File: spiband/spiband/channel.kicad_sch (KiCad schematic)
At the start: 16 parts, among them J2 Conn_01x06, U10 SN74LVC1T45DBV, U11 SN74LVC1T45DBV, U6 TLV70018_SOT353, U8 SN74LVC1T45DBV, U9 SN74LVC1T45DBV

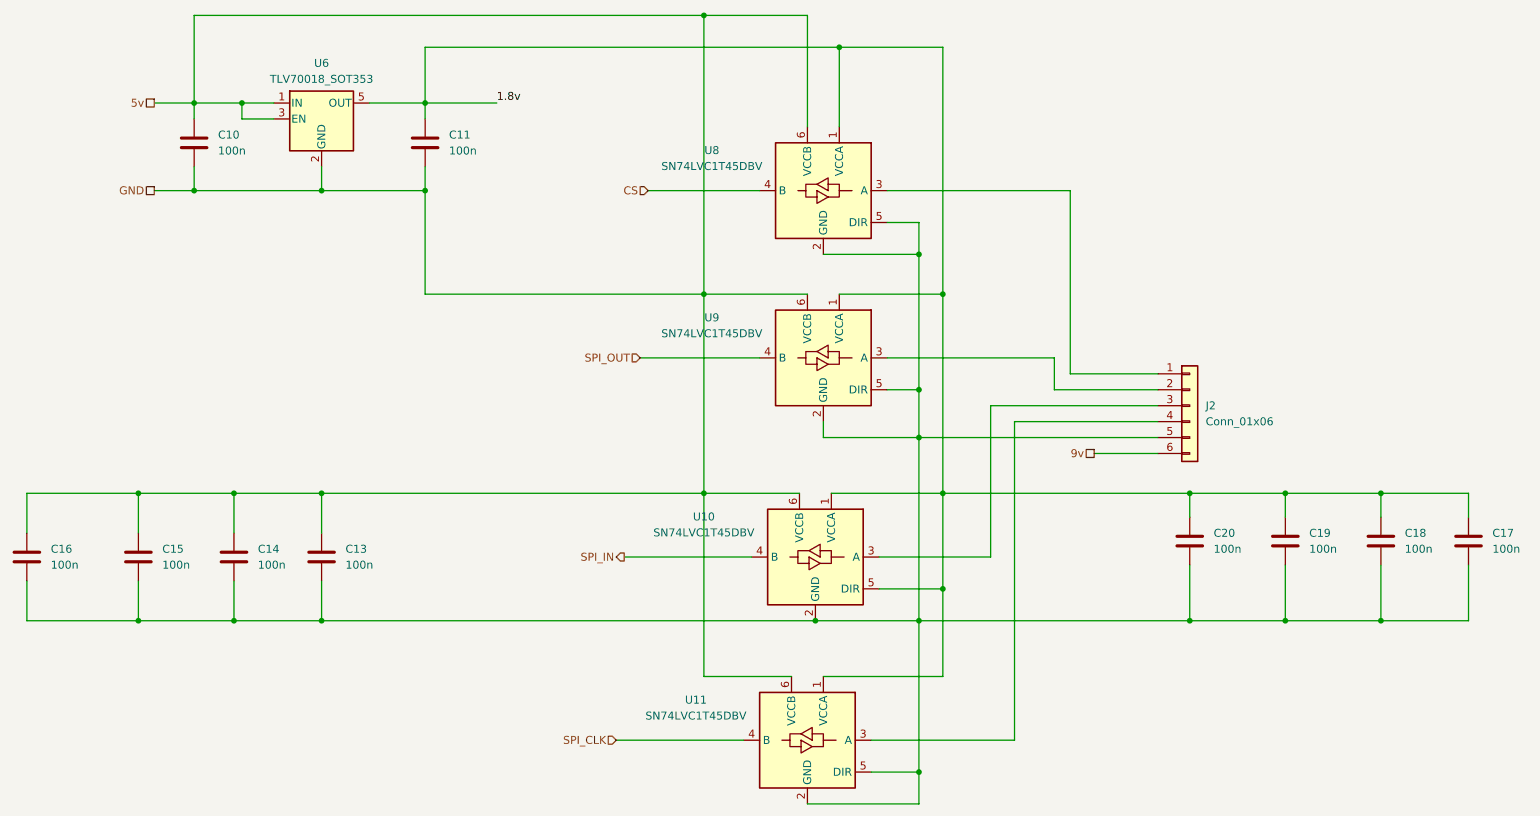
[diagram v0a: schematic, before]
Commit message: SPI band schema done.
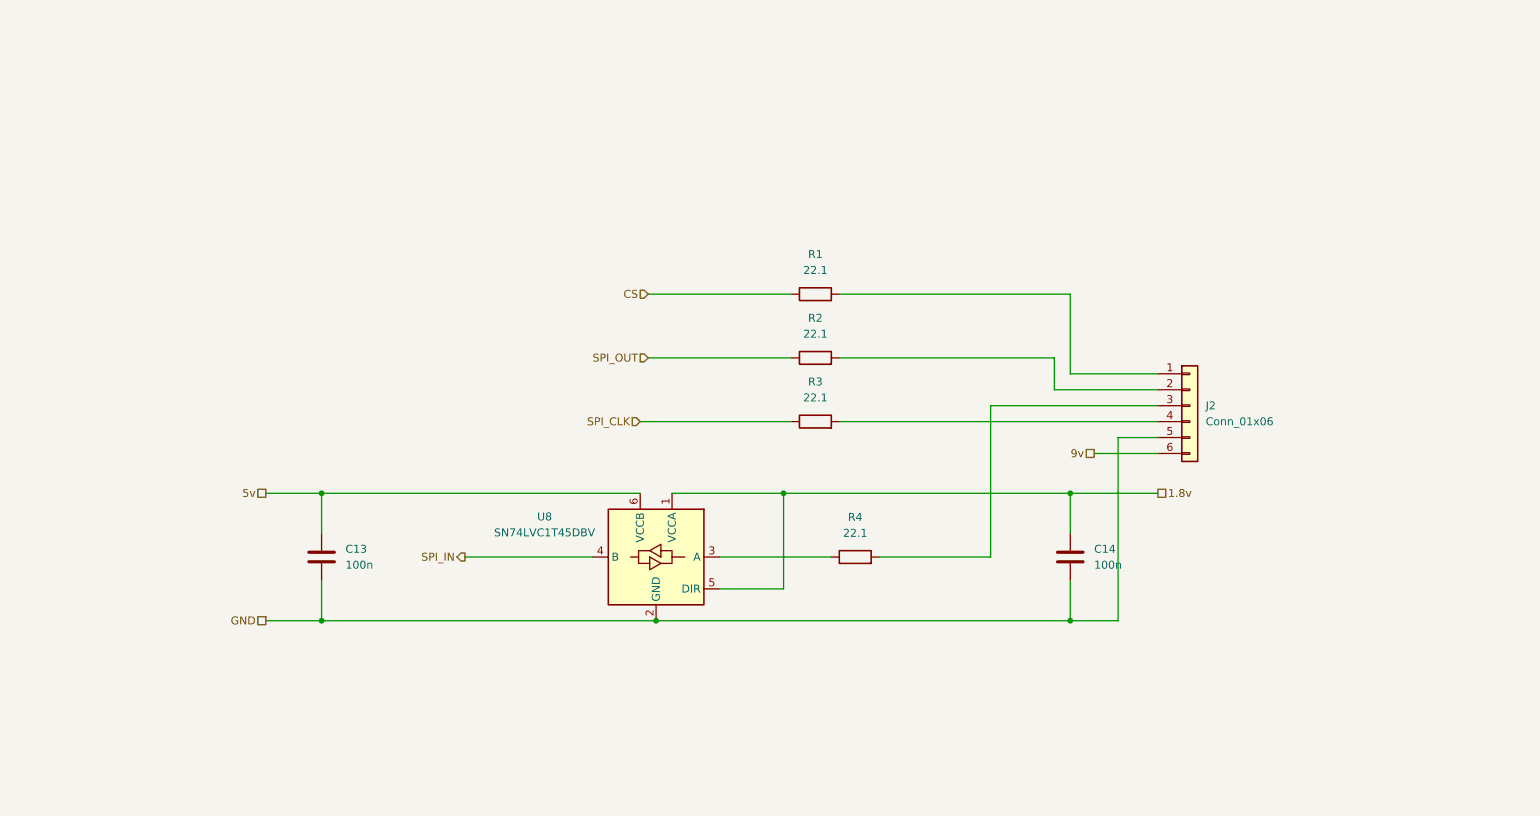
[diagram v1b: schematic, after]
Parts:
- removed C10, C11, C14, C15, C16, C17, C18, C19: 100n, Capacitor_THT:C_Disc_D4.3mm_W1.9mm_P5.00m, symbol Device:C
- removed U11, U8, U9: SN74LVC1T45DBV, Package_TO_SOT_SMD:SOT-23-6, symbol Logic_LevelTranslator:SN74LVC1T45DBV
- removed U6: TLV70018_SOT353, Package_TO_SOT_SMD:SOT-353_SC-70-5, symbol Regulator_Linear:TLV70018_SOT353
- added R1, R2, R3, R4: 22.1, Resistor_SMD:R_0805_2012Metric_Pad1.20x1.40mm_HandSolder, symbol Device:R
- C13: footprint Capacitor_THT:C_Disc_D4.3mm_W1.9mm_P5.00m -> Capacitor_SMD:C_0402_1005Metric_Pad0.74x0.62mm_HandSolder
- C14: renamed from C20; footprint Capacitor_THT:C_Disc_D4.3mm_W1.9mm_P5.00m -> Capacitor_SMD:C_0402_1005Metric_Pad0.74x0.62mm_HandSolder
- renumbered U10 to U8
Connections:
- net CS: now also R1.1
- net SPI_CLK: now also R3.1
- net SPI_OUT: now also R2.1
- net GND: now reaches C13.2, C14.2, J2.5 (Pin_5), U8.2 (GND)
- net at J2.1 (Pin_1): now also R1.2
- net at U8.3 (A): now also R4.1; no longer J2.3 (Pin_3)
- net at J2.2 (Pin_2): now also R2.2
- net at J2.4 (Pin_4): now also R3.2
- new net: J2.3 (Pin_3), R4.2
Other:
- moved on the sheet: C14, U8
